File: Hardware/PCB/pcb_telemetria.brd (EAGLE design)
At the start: 77.5 x 104.1 mm, 33 parts

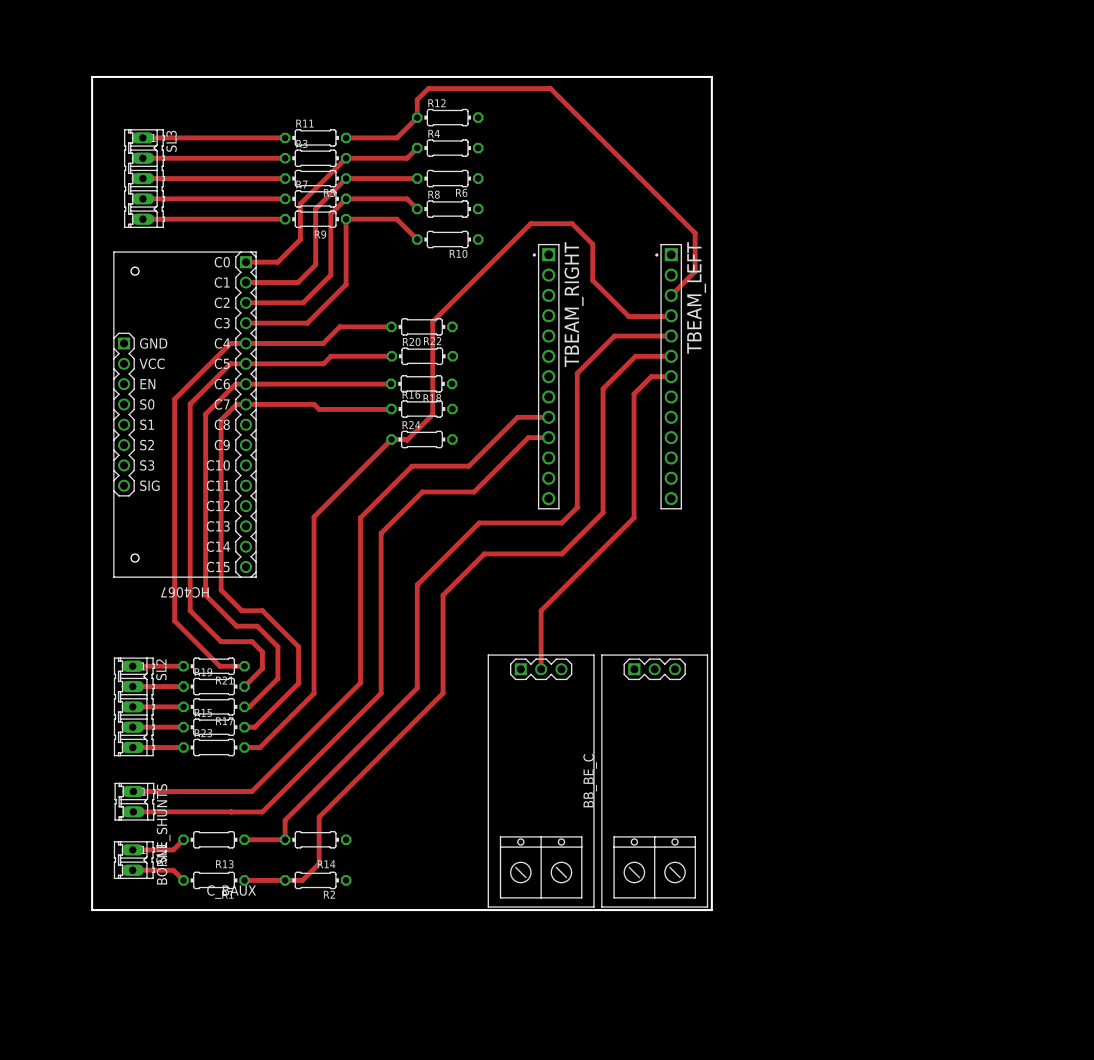
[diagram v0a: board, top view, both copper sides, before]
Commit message: Limpeza e mudanca dos nomes
Update de organizacao
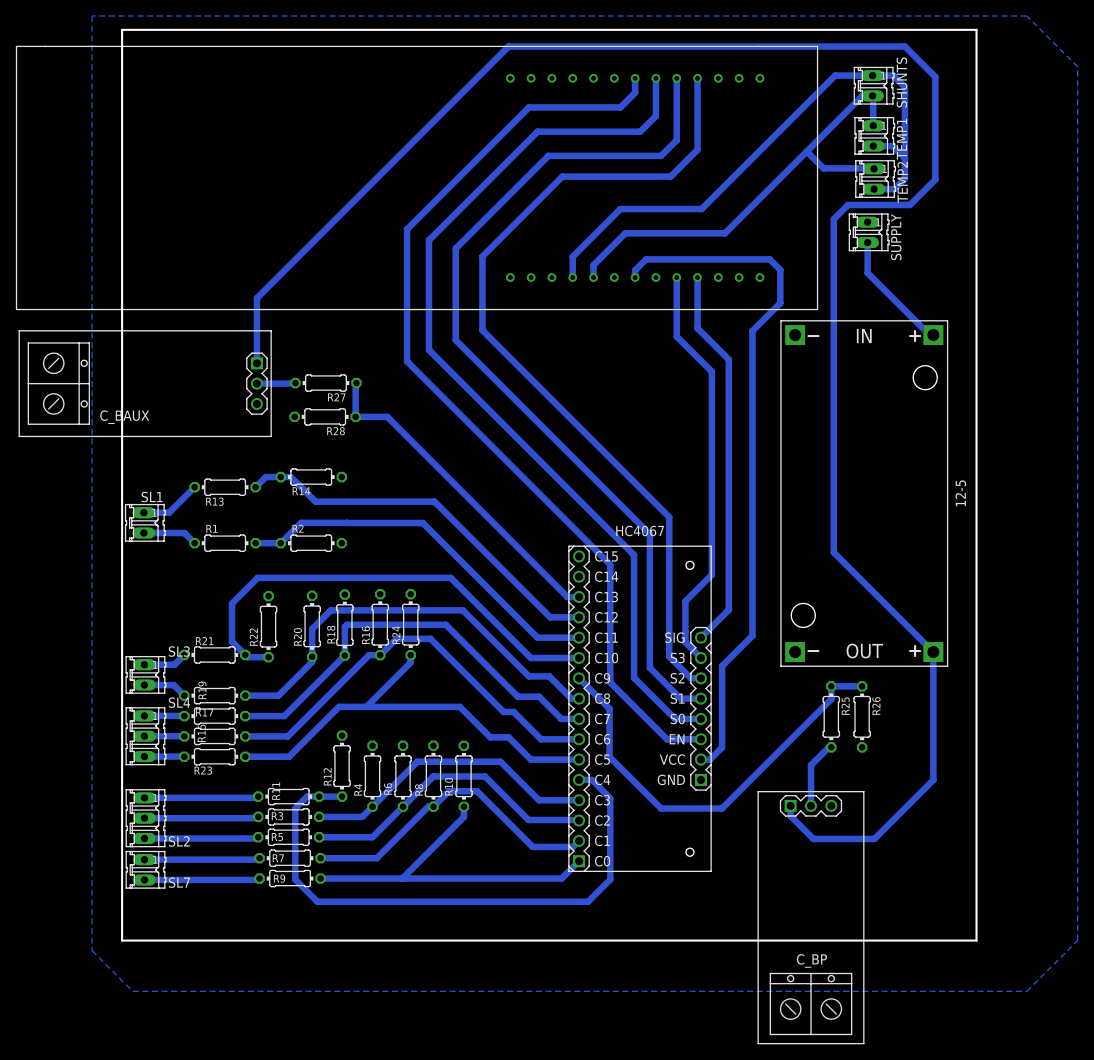
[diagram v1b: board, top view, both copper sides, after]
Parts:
- removed BB_BE_C: CURRENT-SENSOR-ACS712, diy-modules:CURRENT-SENSOR-ACS712
- removed BORNE_SHUNTS: (no value), con-amp-quick:02P
- removed TBEAM_LEFT, TBEAM_RIGHT: 61301311121, Headers:61301311121
- added 12-5: DC-DC-STEP-DOWN-LM2596, diy-modules:DC-DC-STEP-DOWN-LM2596
- added C_BP: CURRENT-SENSOR-ACS712, diy-modules:CURRENT-SENSOR-ACS712
- added R25, R27: 2.2k, rcl:0204/7
- added R26, R28: 3.9k, rcl:0204/7
- added SHUNTS, SL7, SUPPLY, TEMP1, TEMP2: (no value), con-amp-quick:02P
- added SL4: (no value), con-amp-quick:03P
- added U$1: TTGOBEAM, bibliotecattgo:TTGOBEAM
- SL2: device con-amp-quick:05P -> con-amp-quick:03P
- SL3: device con-amp-quick:05P -> con-amp-quick:02P
- moved R7 82.5 mm to (24.7, 6.48)
- moved R9 82.5 mm to (24.7, 3.94)
- moved R11 82.4 mm to (24.6, 14.2)
- moved R3 82.4 mm to (24.6, 11.6)
- moved R5 82.4 mm to (24.6, 9.10)
- moved R12 82.1 mm to (31.2, 18.0), turned to 90 degrees
- moved R4 79.1 mm to (35.1, 16.7), turned to 90 degrees
- moved R6 74.9 mm to (38.9, 16.7), turned to 270 degrees
- moved R8 70.9 mm to (42.7, 16.7), turned to 90 degrees
- moved C_BAUX 70.1 mm to (6.63, 65.8), turned to 0 degrees
- moved HC4067 67.7 mm to (68.5, 25.2), turned to 0 degrees
- moved R10 67.1 mm to (46.5, 16.7), turned to 270 degrees
- moved SL3 62.0 mm to (6.54, 29.4)
- moved R14 45.3 mm to (27.4, 54.1)
- moved R13 44.1 mm to (16.6, 52.9)
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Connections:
- removed net EN: HC4067.J2.3
- removed net S0: HC4067.J2.4
- removed net S1: HC4067.J2.5
- removed net S2: HC4067.J2.6
- removed net S3: HC4067.J2.7
- removed net SIG: HC4067.J2.8
- new net GND1: U$1.GND1
- new net GND2: U$1.GND3
- new net N$1: C_BP.2, R25.2
- new net N$2: C_BAUX.2, R27.2
- new net VI: 12-5.IN+, SUPPLY.2
- net 0: now also HC4067.J2.7, U$1.0; no longer TBEAM_RIGHT.5
- net 13: now also U$1.13; no longer R23.2, R24.1, TBEAM_LEFT.4
- net 14: now also U$1.14; no longer R13.1, R14.2, TBEAM_LEFT.5
- net 2: now also U$1.2; no longer R11.2, R12.1, TBEAM_LEFT.3
- net 21: now also SHUNTS.1, TEMP1.2, TEMP2.2, U$1.21; no longer BORNE_SHUNTS.2, TBEAM_RIGHT.10
- net 22: now also SHUNTS.2, TEMP1.1, TEMP2.1, U$1.22; no longer BORNE_SHUNTS.1, TBEAM_RIGHT.9
- net 23: now also U$1.23; no longer TBEAM_RIGHT.3
- net 25: now also U$1.25; no longer R1.1, R2.2, TBEAM_LEFT.6
- net 3.3V: now also U$1.3.3V; no longer TBEAM_RIGHT.11
- net 32: now also HC4067.J2.4, U$1.32; no longer TBEAM_LEFT.8
- net 33: now also HC4067.J2.3, U$1.33; no longer C_BAUX.2, TBEAM_LEFT.7
- net 34: now also HC4067.J2.6, U$1.34; no longer TBEAM_LEFT.10
- net 35: now also HC4067.J2.5, U$1.35; no longer TBEAM_LEFT.9
- net 3V3: now also HC4067.J2.2, U$1.3V3; no longer TBEAM_RIGHT.7
- net 4: now also HC4067.J2.8, U$1.4; no longer TBEAM_RIGHT.4
- net 5V: now also U$1.5V; no longer TBEAM_LEFT.1
- net BAT_AUX: now also R21.2, SL3.1; no longer R23.1, SL2.5
- net BB_IN: now also SL4.2; no longer SL2.4
- net BE_IN: now also SL4.1; no longer SL2.3
- net BTN_CRUZEIRO: now also SL7.2; no longer SL3.5
- net BTN_RE: now also SL2.3; no longer SL3.3
- net C0: now also R10.2, R9.1; no longer R3.2, R4.1
- net C1: now also R7.2, R8.1; no longer R5.1, R6.2
- net C10: now also R21.1, R22.2
- net C11: now also R1.1, R2.2
- net C12: now also R13.1, R14.2
- net C13: now also R27.1, R28.1
- net C2: now also R5.1, R6.2; no longer R7.2, R8.1
- net C3: now also R3.2, R4.1; no longer R10.2, R9.1
- net C4: now also R11.2, R12.1; no longer R21.1, R22.2
- net C5: now also R23.2, R24.1; no longer R19.2, R20.1
- net C6: now also R15.2, R16.1; no longer R17.1, R18.2
- net C7: now also R17.1, R18.2; no longer R15.2, R16.1
- net C8: now also R19.2, R20.1
- net C9: now also R25.1, R26.1
- net COOLER_D: now also SL3.2; no longer SL2.2
- net COOLER_E: now also R23.1, SL4.3; no longer R21.2, SL2.1
- net DMS_IN: now also SL2.2; no longer SL3.2
- net GND: now also 12-5.IN-, 12-5.OUT-, C_BP.3, R26.2, R28.2, SUPPLY.1, U$1.GND; no longer BB_BE_C.3, TBEAM_LEFT.2, TBEAM_RIGHT.6, TBEAM_RIGHT.8
- net LORA1: now also U$1.LORA1; no longer TBEAM_RIGHT.13
- net LORA2: now also U$1.LORA2; no longer TBEAM_RIGHT.12
- net ON-OFF_MOTOR: now also SL7.1; no longer SL3.4
- net POT_IN: now also SL2.1; no longer SL3.1
- net RST: now also U$1.RST; no longer TBEAM_LEFT.11
- net RX: now also U$1.RX; no longer TBEAM_RIGHT.2
- net TX: now also U$1.TX; no longer TBEAM_RIGHT.1
- net VCC: now also 12-5.OUT+, C_BP.1; no longer BB_BE_C.1, HC4067.J2.2
- net VN: now also U$1.VN; no longer TBEAM_LEFT.12
- net VP: now also U$1.VP; no longer TBEAM_LEFT.13
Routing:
- net VCC: track 0.00 -> 233.7 mm
- net 32: track 0.00 -> 115.3 mm
- net 35: track 0.00 -> 111.4 mm
- net 13: track 107.8 -> 0.00 mm
- net 34: track 0.00 -> 106.1 mm
- net 25: track 100.1 -> 0.00 mm
- net 14: track 98.2 -> 0.00 mm
- net 3V3: track 0.00 -> 86.1 mm
- net 33: track 44.8 -> 118.8 mm
- net 2: track 64.0 -> 0.00 mm
- net C10: track 0.00 -> 59.0 mm
- net C8: track 0.00 -> 53.1 mm
- net C9: track 0.00 -> 52.9 mm
- net 0: track 0.00 -> 51.5 mm
- net C12: track 0.00 -> 48.2 mm
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- added copper zone on layer 16, net GND
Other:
- board size 77.5 x 104.1 mm -> 106.8 x 113.8 mm
